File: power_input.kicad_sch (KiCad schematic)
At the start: 26 parts, among them J4 12V -, J5 12V +, Q1 AONR21321, U11 XC6206PxxxMR, U6 TPS565242

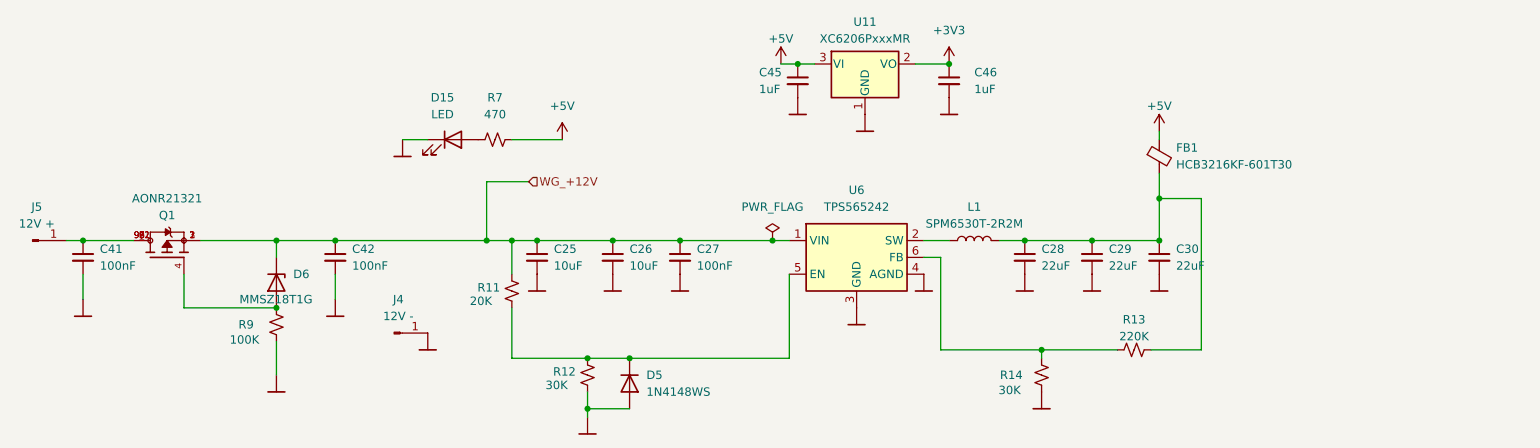
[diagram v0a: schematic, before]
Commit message: new buck
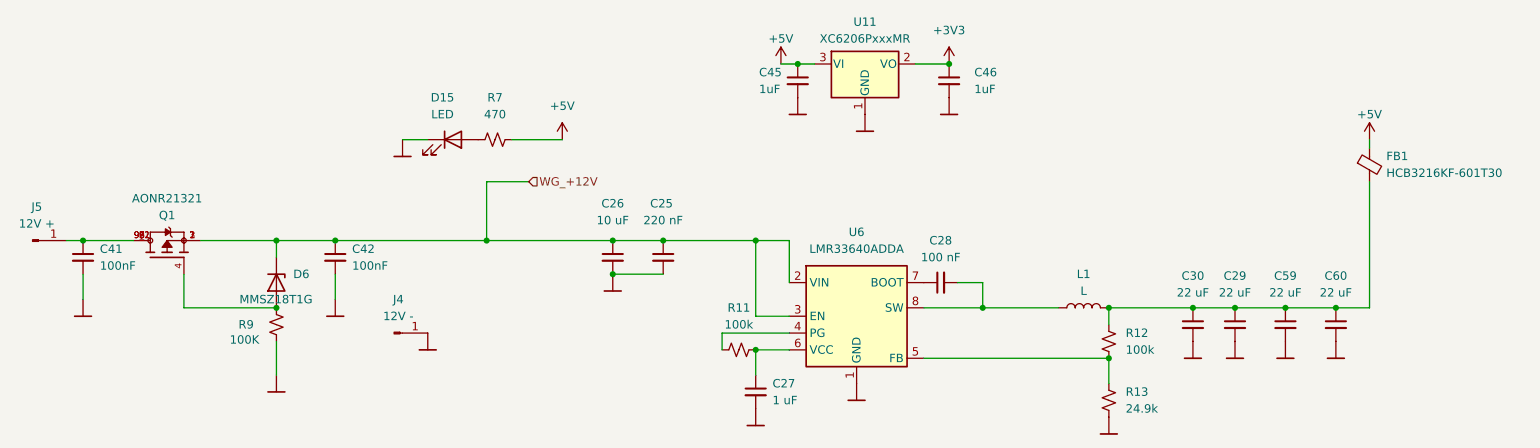
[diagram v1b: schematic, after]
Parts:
- removed D5: 1N4148WS, Diode_SMD:D_SOD-323, symbol Diode:1N4148WS
- removed R14: 30K, Resistor_SMD:R_0603_1608Metric, symbol Device:R_Small_US
- removed U6: TPS565242, Package_TO_SOT_SMD:SOT6_DRL_TEX-L, symbol Regulator_Switching:TPS565242
- added C59, C60: 22 uF, symbol Device:C_Small
- added U6: LMR33640ADDA, Package_SO:Texas_HSOP-8-1EP_3.9x4.9mm_P1.27mm_ThermalVias, symbol Regulator_Switching:LMR33640ADDA
- C25: value 10uF -> 220 nF
- C26: value 10uF -> 10 uF
- C27: value 100nF -> 1 uF
- C28: value 22uF -> 100 nF; footprint Capacitor_SMD:C_0603_1608Metric -> (none)
- C29, C30: value 22uF -> 22 uF; footprint Capacitor_SMD:C_0603_1608Metric -> (none)
- L1: value SPM6530T-2R2M -> L; footprint Inductor_SMD:IND_SPM6530T-2R2M -> (none)
- R11: value 20K -> 100k
- R12: value 30K -> 100k; footprint Resistor_SMD:R_0603_1608Metric -> (none)
- R13: value 220K -> 24.9k; footprint Resistor_SMD:R_0603_1608Metric -> (none)
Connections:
- net WG_+12V: now also U6.2 (VIN), U6.3 (EN); no longer C27.1, R11.1
- net at C29.1, C30.1, FB1.2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: now also R12.1, C59.1, C60.1; no longer C28.1, R13.2
- net at L1.1: now also C28.2, U6.8 (SW)
- net at R11.2: now also C27.1, U6.6 (VCC); no longer R12.1
- net at R13.1: now also R12.2, U6.5 (FB)
- net at C26.2: now also C25.2
- new net: U6.1 (GND), U6.9 (GND)
- new net: R11.1, U6.4 (PG)
- new net: C28.1, U6.7 (BOOT)
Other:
- moved on the sheet: FB1
